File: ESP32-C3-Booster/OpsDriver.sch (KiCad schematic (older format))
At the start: 14 parts, among them U501 DRV8873HPWPR

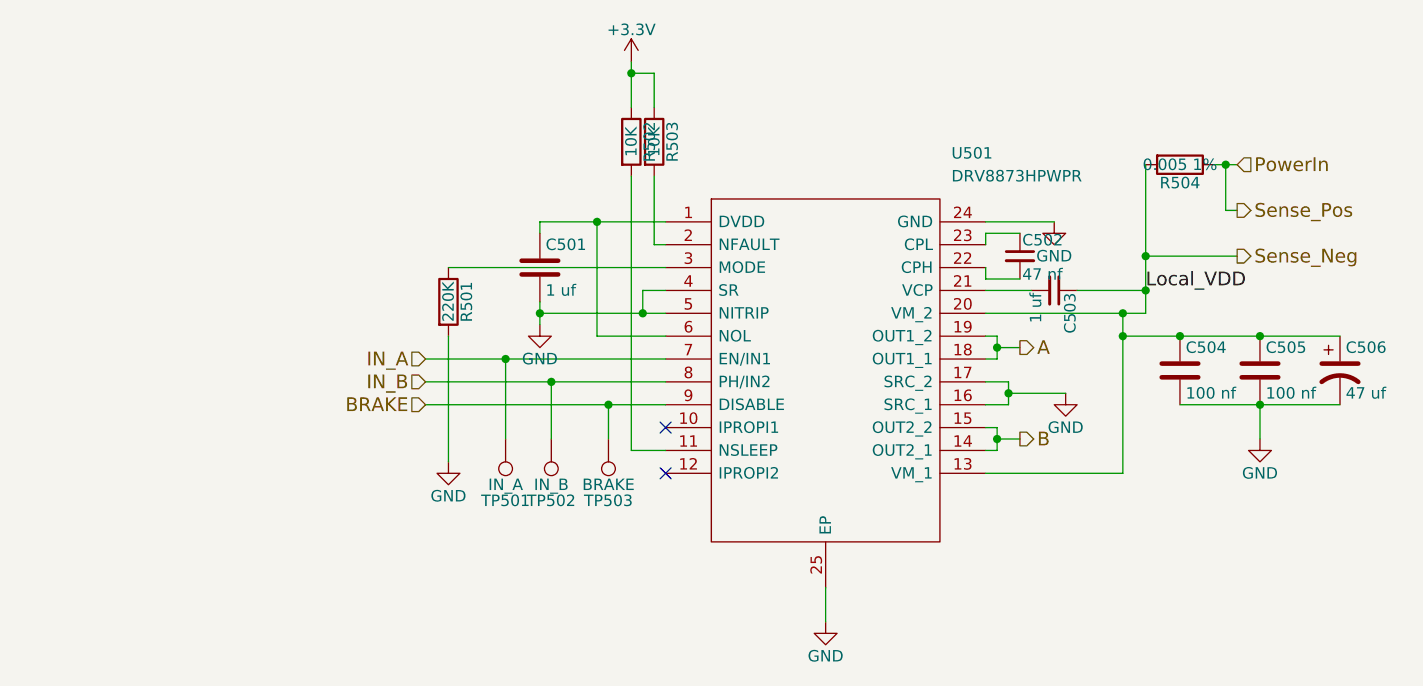
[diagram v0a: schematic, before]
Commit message: Completed first pass ESP32-C3-Booster.
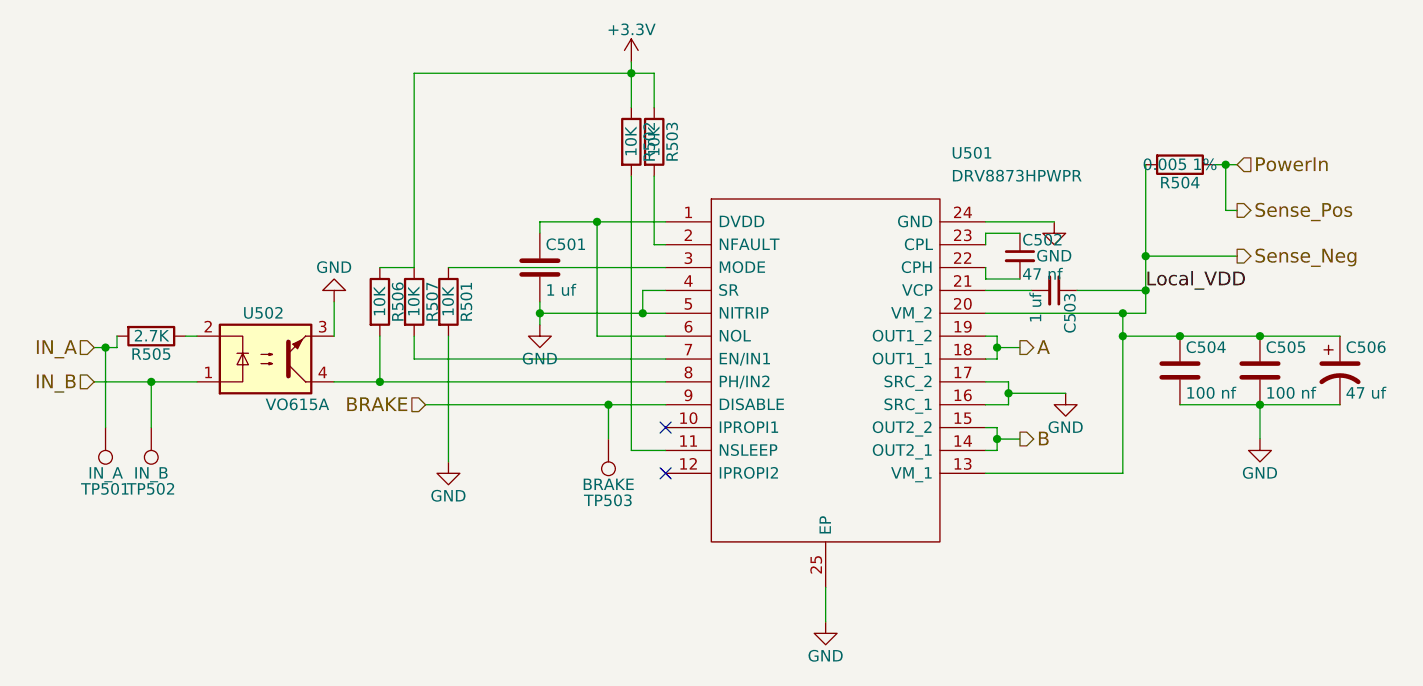
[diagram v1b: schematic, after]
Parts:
- added R505: 2.7K, Resistors_SMD:R_0603, symbol R
- added R506, R507: 10K, Resistors_SMD:R_0603, symbol R
- added U502: VO615A, Housings_SOIC:SO-4_7.6x3.6mm_Pitch2.54mm, symbol VO615A
- R501: value 220K -> 10K; Mouser Part Number 279-CRGCQ0603F220K -> 279-CRGCQ0603F10K
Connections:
- net +3V3: now also R506.1, R507.1
- net GND: now also U502.3
- net IN_A: now also R505.2; no longer U501.7 (EN/IN1)
- net IN_B: now also U502.1; no longer U501.8 (PH/IN2)
- new net: R507.2, U501.7 (EN/IN1)
- new net: R506.2, U501.8 (PH/IN2), U502.4
- new net: R505.1, U502.2
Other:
- moved on the sheet: TP501, TP502
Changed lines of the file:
@@
 LIBS:mcp9701at
 LIBS:MCP9700T-E_LT
+LIBS:ina180b
 LIBS:ESP32-C3-Booster-cache
 EELAYER 25 0
@@
 Comment4 ""
 $EndDescr
-Text HLabel 2500 2500 0    60   Input ~ 0
+Text HLabel 1050 2500 0    60   Input ~ 0
 IN_B
-Text HLabel 2500 2400 0    60   Input ~ 0
+Text HLabel 1050 2350 0    60   Input ~ 0
 IN_A
 Text HLabel 2500 2600 0    60   Input ~ 0
@@
 Sense_Neg
 $Comp
-L GND #PWR505
+L GND #PWR043
 U 1 1 630A7E57
 P 5250 1800
-F 0 "#PWR505" H 5250 1550 50  0001 C CNN
+F 0 "#PWR043" H 5250 1550 50  0001 C CNN
 F 1 "GND" H 5250 1650 50  0000 C CNN
 F 2 "" H 5250 1800 50  0001 C CNN
@@
 $EndComp
 $Comp
-L GND #PWR504
+L GND #PWR044
 U 1 1 630A7E58
 P 4250 3550
-F 0 "#PWR504" H 4250 3300 50  0001 C CNN
+F 0 "#PWR044" H 4250 3300 50  0001 C CNN
 F 1 "GND" H 4250 3400 50  0000 C CNN
 F 2 "" H 4250 3550 50  0001 C CNN
@@
 $EndComp
 $Comp
-L GND #PWR507
+L GND #PWR045
 U 1 1 630A7E5F
 P 6150 2750
-F 0 "#PWR507" H 6150 2500 50  0001 C CNN
+F 0 "#PWR045" H 6150 2500 50  0001 C CNN
 F 1 "GND" H 6150 2600 50  0000 C CNN
 F 2 "" H 6150 2750 50  0001 C CNN
@@
 $EndComp
 $Comp
-L GND #PWR506
+L GND #PWR046
 U 1 1 630A7E60
 P 5300 2550
-F 0 "#PWR506" H 5300 2300 50  0001 C CNN
+F 0 "#PWR046" H 5300 2300 50  0001 C CNN
 F 1 "GND" H 5300 2400 50  0000 C CNN
 F 2 "" H 5300 2550 50  0001 C CNN
@@
 $EndComp
 $Comp
-L GND #PWR502
+L GND #PWR047
 U 1 1 630A7E62
 P 3000 2250
-F 0 "#PWR502" H 3000 2000 50  0001 C CNN
+F 0 "#PWR047" H 3000 2000 50  0001 C CNN
 F 1 "GND" H 3000 2100 50  0000 C CNN
 F 2 "" H 3000 2250 50  0001 C CNN
@@
 $EndComp
 $Comp
-L +3.3V #PWR503
+L +3.3V #PWR048
 U 1 1 630A7E65
 P 3400 1100
-F 0 "#PWR503" H 3400 950 50  0001 C CNN
+F 0 "#PWR048" H 3400 950 50  0001 C CNN
 F 1 "+3.3V" H 3400 1240 50  0000 C CNN
 F 2 "" H 3400 1100 50  0001 C CNN
@@
 P 2600 2150
 F 0 "R501" V 2680 2150 50  0000 C CNN
-F 1 "220K" V 2600 2150 50  0000 C CNN
+F 1 "10K" V 2600 2150 50  0000 C CNN
 F 2 "Resistors_SMD:R_0603" V 2530 2150 50  0001 C CNN
 F 3 "" H 2600 2150 50  0001 C CNN
-F 4 "279-CRGCQ0603F220K " V 2600 2150 60  0001 C CNN "Mouser Part Number"
+F 4 "279-CRGCQ0603F10K " V 2600 2150 60  0001 C CNN "Mouser Part Number"
 	1    2600 2150
 	1    0    0    -1
 $EndComp
 $Comp
-L GND #PWR501
+L GND #PWR049
 U 1 1 630A7E67
 P 2600 2850
-F 0 "#PWR501" H 2600 2600 50  0001 C CNN
+F 0 "#PWR049" H 2600 2600 50  0001 C CNN
 F 1 "GND" H 2600 2700 50  0000 C CNN
 F 2 "" H 2600 2850 50  0001 C CNN
@@
 L TEST_1P TP502
 U 1 1 630A7E69
-P 3050 2750
-F 0 "TP502" H 3050 3020 50  0000 C CNN
-F 1 "IN_B" H 3050 2950 50  0000 C CNN
-F 2 "Measurement_Points:Measurement_Point_Round-SMD-Pad_Big" H 3250 2750 50  0001 C CNN
-F 3 "" H 3250 2750 50  0001 C CNN
-	1    3050 2750
+P 1300 2700
+F 0 "TP502" H 1300 2970 50  0000 C CNN
+F 1 "IN_B" H 1300 2900 50  0000 C CNN
+F 2 "Measurement_Points:Measurement_Point_Round-SMD-Pad_Big" H 1500 2700 50  0001 C CNN
+F 3 "" H 1500 2700 50  0001 C CNN
+	1    1300 2700
 	-1   0    0    1
 $EndComp
@@
 L TEST_1P TP501
 U 1 1 630A7E6A
-P 2850 2750
-F 0 "TP501" H 2850 3020 50  0000 C CNN
-F 1 "IN_A" H 2850 2950 50  0000 C CNN
-F 2 "Measurement_Points:Measurement_Point_Round-SMD-Pad_Big" H 3050 2750 50  0001 C CNN
-F 3 "" H 3050 2750 50  0001 C CNN
-	1    2850 2750
+P 1100 2700
+F 0 "TP501" H 1100 2970 50  0000 C CNN
+F 1 "IN_A" H 1100 2900 50  0000 C CNN
+F 2 "Measurement_Points:Measurement_Point_Round-SMD-Pad_Big" H 1300 2700 50  0001 C CNN
+F 3 "" H 1300 2700 50  0001 C CNN
+	1    1100 2700
 	-1   0    0    1
 $EndComp
 Wire Wire Line
-	2500 2400 3550 2400
-Wire Wire Line
-	2500 2500 3550 2500
+	2450 2400 3550 2400
+Wire Wire Line
+	2100 2500 3550 2500
 Wire Wire Line
 	2500 2600 3550 2600
@@
 	3400 1100 3400 1300
 Wire Wire Line
-	3500 1300 3500 1150
-Wire Wire Line
-	3500 1150 3400 1150
+	3500 1150 3500 1300
+Wire Wire Line
+	2450 1150 3500 1150
 Connection ~ 3400 1150
 Wire Wire Line
@@
 Connection ~ 3000 2200
 Connection ~ 3450 2200
-Wire Wire Line
-	2850 2750 2850 2400
-Connection ~ 2850 2400
-Wire Wire Line
-	3050 2750 3050 2500
-Connection ~ 3050 2500
 Wire Wire Line
 	3300 2750 3300 2600
@@
 	1    0    0    -1
 $EndComp
+Wire Wire Line
+	1050 2500 1500 2500
+Wire Wire Line
+	1300 2500 1300 2700
+Wire Wire Line
+	1050 2350 1150 2350
+Wire Wire Line
+	1100 2350 1100 2700
+$Comp
+L VO615A U502
+U 1 1 630BFB12
+P 1800 2400
+F 0 "U502" H 1700 2200 50  0000 L CNN
+F 1 "VO615A" H 1800 2600 50  0000 L CNN
+F 2 "Housings_SOIC:SO-4_7.6x3.6mm_Pitch2.54mm" H 1600 2200 50  0001 L CIN
+F 3 "" H 1800 2400 50  0001 L CNN
+F 4 "78-VO615A-7X017T" H 1800 2400 60  0001 C CNN "Mouser Part Number"
+	1    1800 2400
+	1    0    0    1
+$EndComp
+$Comp
+L R R507
+U 1 1 630BFBF6
+P 2450 2150
+F 0 "R507" V 2530 2150 50  0000 C CNN
+F 1 "10K" V 2450 2150 50  0000 C CNN
+F 2 "Resistors_SMD:R_0603" V 2380 2150 50  0001 C CNN
+F 3 "" H 2450 2150 50  0001 C CNN
+F 4 "279-CRGCQ0603F10K " V 2450 2150 60  0001 C CNN "Mouser Part Number"
+	1    2450 2150
+	1    0    0    -1
+$EndComp
+Wire Wire Line
+	2450 2300 2450 2400
+Wire Wire Line
+	2450 2000 2450 1150
+$Comp
+L R R506
+U 1 1 630BFE77
+P 2300 2150
+F 0 "R506" V 2380 2150 50  0000 C CNN
+F 1 "10K" V 2300 2150 50  0000 C CNN
+F 2 "Resistors_SMD:R_0603" V 2230 2150 50  0001 C CNN
+F 3 "" H 2300 2150 50  0001 C CNN
+F 4 "279-CRGCQ0603F10K " V 2300 2150 60  0001 C CNN "Mouser Part Number"
+	1    2300 2150
+	1    0    0    -1
+$EndComp
+Wire Wire Line
+	2300 2000 2450 2000
+$Comp
+L R R505
+U 1 1 630C0001
+P 1300 2300
+F 0 "R505" V 1380 2300 50  0000 C CNN
+F 1 "2.7K" V 1300 2300 50  0000 C CNN
+F 2 "Resistors_SMD:R_0603" V 1230 2300 50  0001 C CNN
+F 3 "" H 1300 2300 50  0001 C CNN
+F 4 "603-AC0603FR-132K7L" V 1300 2300 60  0001 C CNN "Mouser Part Number"
+	1    1300 2300
+	0    1    1    0
+$EndComp
+Wire Wire Line
+	1500 2300 1450 2300
+Connection ~ 1300 2500
+Wire Wire Line
+	1150 2350 1150 2300
+Connection ~ 1100 2350
+Wire Wire Line
+	2300 2300 2300 2500
+Connection ~ 2300 2500
+$Comp
+L GND #PWR050
+U 1 1 630C0BE3
+P 2100 2150
+F 0 "#PWR050" H 2100 1900 50  0001 C CNN
+F 1 "GND" H 2100 2000 50  0000 C CNN
+F 2 "" H 2100 2150 50  0001 C CNN
+F 3 "" H 2100 2150 50  0001 C CNN
+	1    2100 2150
+	-1   0    0    1
+$EndComp
+Wire Wire Line
+	2100 2150 2100 2300
 $EndSCHEMATC
